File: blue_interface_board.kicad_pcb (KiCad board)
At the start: 4 copper layers, 70 x 70 mm, 110 parts, among them J1 Conn_01x05, J2 USB_B_Micro, J3 Conn_01x02, J4 Conn_01x02, J5 Conn_ARM_JTAG_SWD_10, J6 Conn_01x03, Q1 MMBT5401LT1G, Q2 Q_NMOS_GDS, Q3 MMBT3904, Q4 Q_NMOS_GDS, Q5 Q_NMOS_GDS, Q6 Q_NMOS_GDS, U1 93LCxxB, U10 LMZ21700SIL, U2 FT232H, U3 ADM2682E, U4 TPD2E2U06, U5 TPD2E2U06, U6 LM5066, U7 STM32L011K4Tx, U8 ti-LM5163, Y1 12MHz

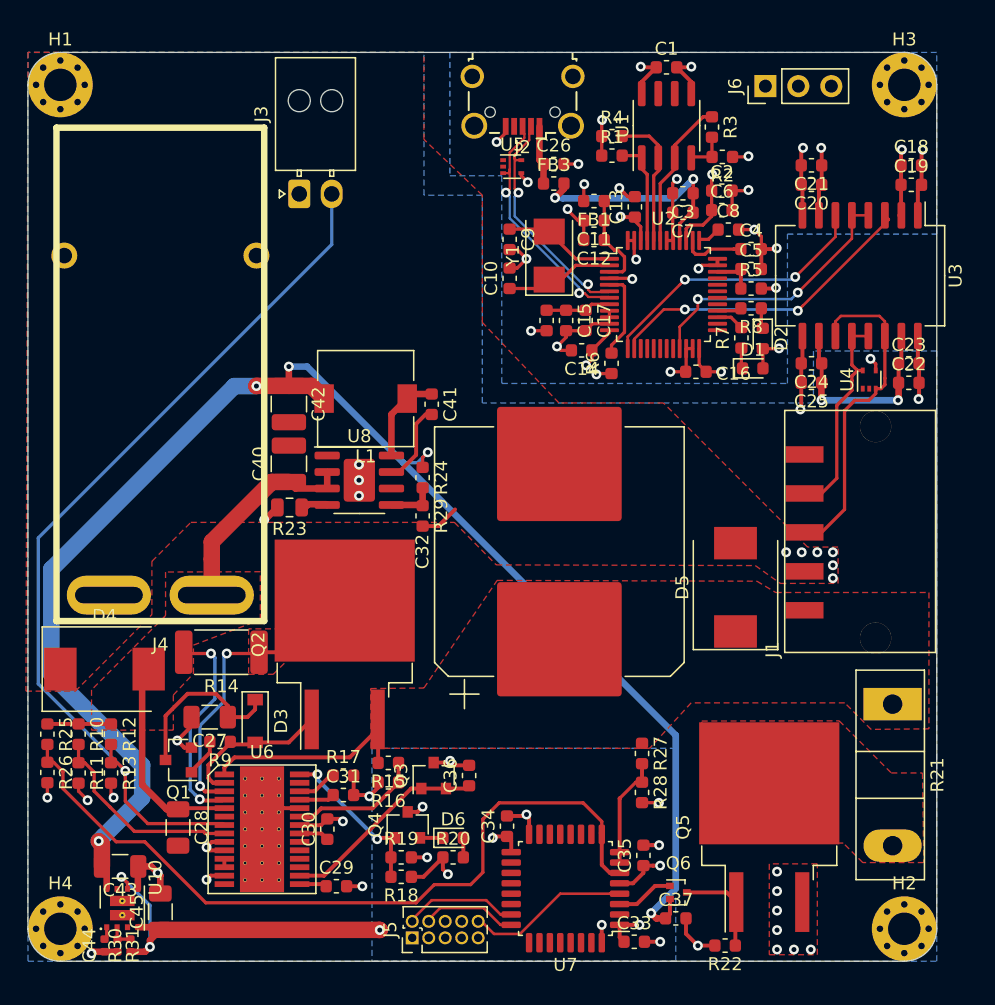
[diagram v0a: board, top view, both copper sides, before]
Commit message: Fix DRCs and minor improvements
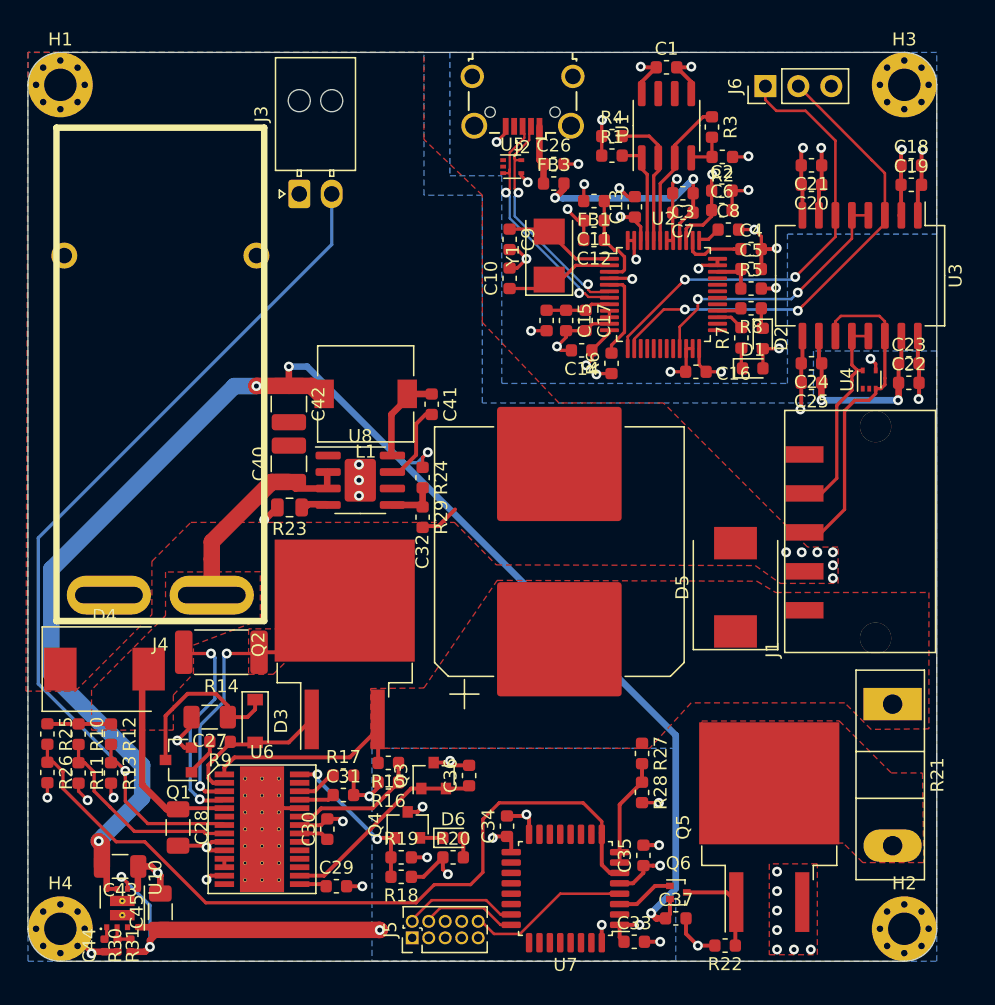
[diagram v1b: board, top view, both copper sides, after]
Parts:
- moved L1 0.37 mm to (115.0, 85.3)
- moved R29 0.10 mm to (119.4, 94.8)
- moved U8 0.07 mm to (114.6, 92.0)
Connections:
- H3 pad 1: GNDPWR -> Net-(H3-Pad1)
- J6 pad 1: /Comms/RS485_A -> /Comms/RS485_TX
- J6 pad 2: /Comms/RS485_B -> /Comms/RS485_RX
- J6 pad 3: GNDPWR -> GNDD
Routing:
- net /Comms/RS485_TX: track 21.7 -> 35.3 mm
- net /Comms/RS485_RX: track 24.7 -> 37.1 mm
- net GNDPWR: track 65.3 -> 70.8 mm
- net +12V: track 120.5 -> 121.3 mm
